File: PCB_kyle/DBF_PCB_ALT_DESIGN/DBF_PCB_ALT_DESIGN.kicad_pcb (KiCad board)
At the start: 4 copper layers, 6 parts

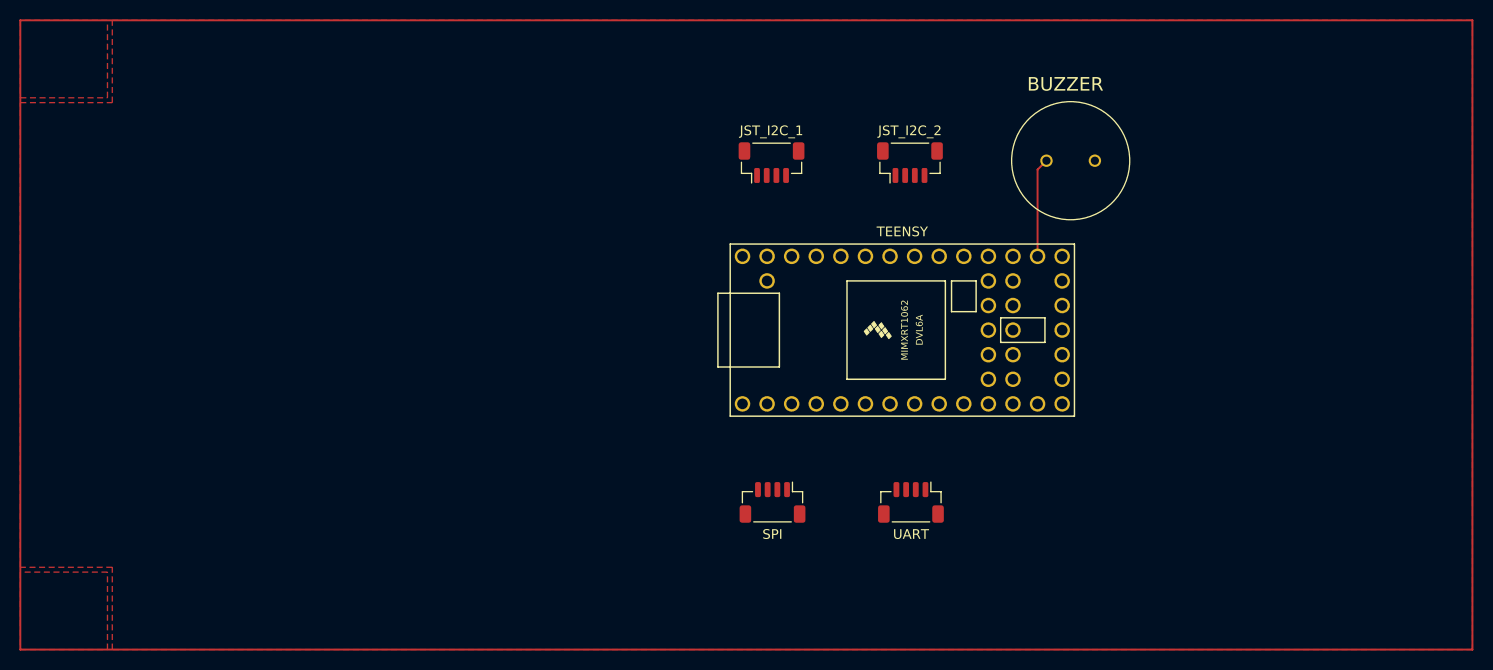
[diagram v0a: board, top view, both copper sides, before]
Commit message: tracing almost complete(?)
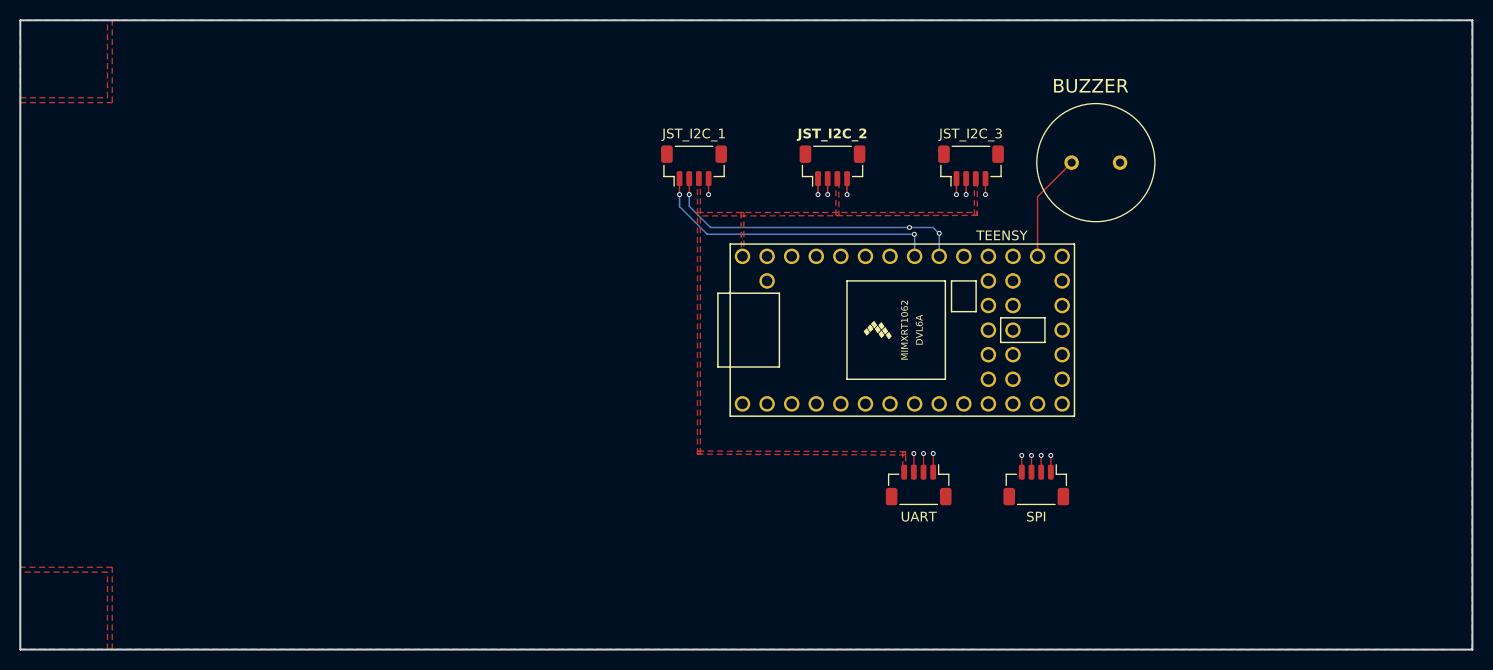
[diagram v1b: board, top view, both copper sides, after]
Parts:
- added JST_I2C_1: JST_SH_BM04B-SRSS-TB_1x04-1MP_P1.00mm_Vertical, Connector_JST:JST_SH_BM04B-SRSS-TB_1x04-1MP_P1.00mm_Vertical, F.Cu at (169.6, 65.0)
- moved UART 15.2 mm to (192.8, 98.0)
- moved SPI 13.1 mm to (204.9, 98.0)
- moved JST_I2C_2 6.31 mm to (183.9, 65.0)
- moved JST_I2C_3 6.31 mm to (198.2, 65.0)
- moved BUZZER 2.61 mm to (211.1, 64.7)
- renumbered JST_I2C_1 to JST_I2C_2, JST_I2C_2 to JST_I2C_3, UART to SPI, SPI to UART
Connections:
- JST_I2C_2 pad 1: (no net) -> SCL0
- JST_I2C_2 pad 2: (no net) -> SDA0
- JST_I2C_2 pad 3: (no net) -> 5V_PWR
- JST_I2C_2 pad 4: (no net) -> GND
- JST_I2C_3 pad 1: (no net) -> SCL0
- JST_I2C_3 pad 2: (no net) -> SDA0
- JST_I2C_3 pad 3: (no net) -> 5V_PWR
- JST_I2C_3 pad 4: (no net) -> GND
- SPI pad 1: (no net) -> SCK
- SPI pad 2: (no net) -> MISO
- SPI pad 3: (no net) -> MOSI
- SPI pad 4: (no net) -> CS
- TEENSY pad 1: (no net) -> GND
- TEENSY pad 10: (no net) -> TX2
- TEENSY pad 12: (no net) -> CS
- TEENSY pad 13: (no net) -> MOSI
- TEENSY pad 14: (no net) -> MISO
- TEENSY pad 20: (no net) -> SCK
- TEENSY pad 25: (no net) -> SDA0
- TEENSY pad 26: (no net) -> SCL0
- TEENSY pad 32: (no net) -> GND
- TEENSY pad 33: (no net) -> 5V_PWR
- TEENSY pad 9: (no net) -> RX2
- UART pad 1: (no net) -> TX2
- UART pad 2: (no net) -> RX2
- UART pad 3: (no net) -> GND
- UART pad 4: (no net) -> 5V_PWR
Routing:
- net SCL0: track 0.00 -> 54.0 mm, vias 0 -> 4
- net SDA0: track 0.00 -> 52.2 mm, vias 0 -> 5
- net SCK: track 0.00 -> 24.4 mm, vias 0 -> 1
- net TX2: track 0.00 -> 8.36 mm, vias 0 -> 1
- net CS: track 0.00 -> 8.09 mm, vias 0 -> 1
- net MISO: track 0.00 -> 7.95 mm, vias 0 -> 1
- net RX2: track 0.00 -> 7.73 mm, vias 0 -> 1
- net MOSI: track 0.00 -> 7.32 mm, vias 0 -> 1
- net GND: track 0.00 -> 6.88 mm, vias 0 -> 4
- net buzzer: track 10.3 -> 11.1 mm
- added copper zone on B.Cu, net (none)
- added copper zone on In2.Cu, net (none)
- added copper zone on F.Cu, net 5V_PWR
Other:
- board outline added: 150 x 65 mm
